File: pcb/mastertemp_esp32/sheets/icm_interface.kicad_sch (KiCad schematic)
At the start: 9 parts, among them J2 OPERATING_CONTROL_7P, K1 G5Q-1A-DC5_CANDIDATE, K2 G5Q-1A-DC5_CANDIDATE, Q1 RELAY_K1_LOW_SIDE_TBD, Q2 RELAY_K2_LOW_SIDE_TBD

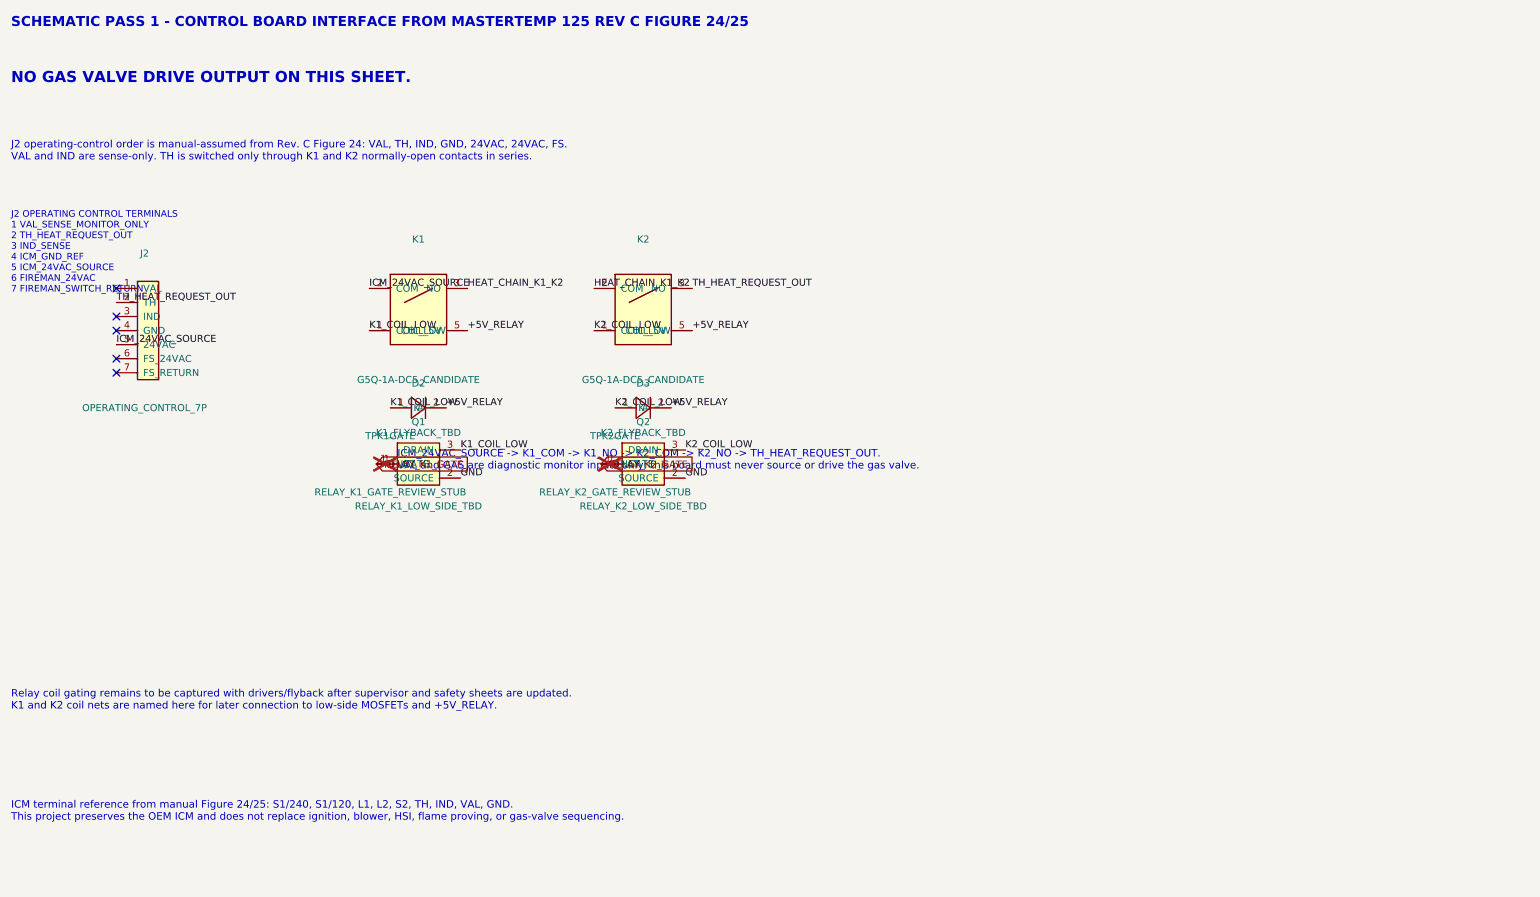
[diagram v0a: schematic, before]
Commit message: AI
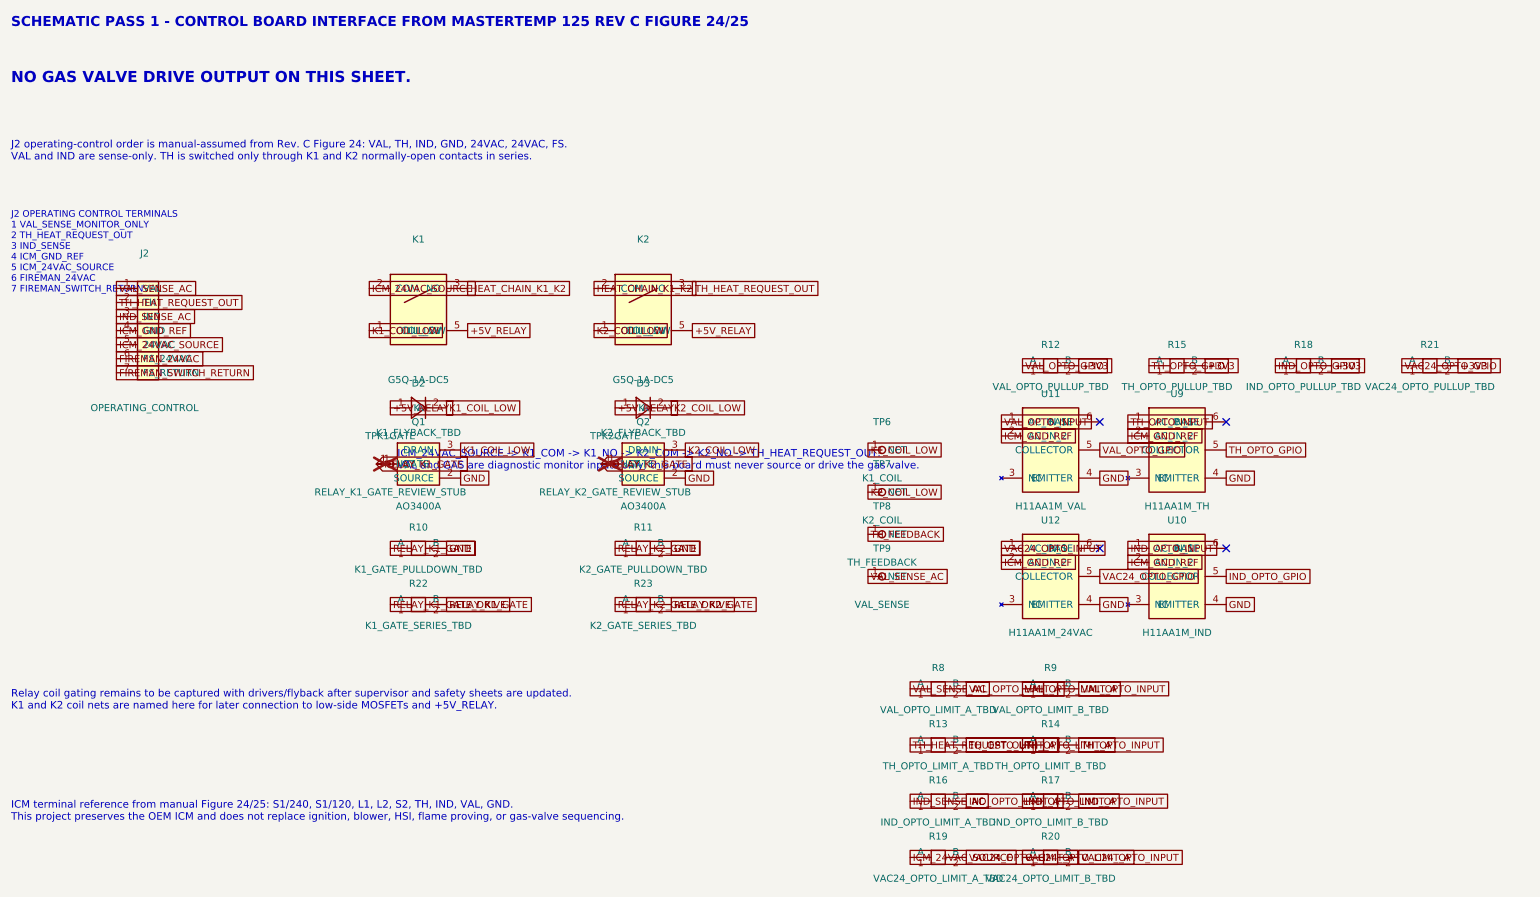
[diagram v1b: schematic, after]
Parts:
- added R10: K1_GATE_PULLDOWN_TBD, Resistor_SMD:R_0805_2012Metric, symbol mastertemp_esp32:Resistor_2pin
- added R11: K2_GATE_PULLDOWN_TBD, Resistor_SMD:R_0805_2012Metric, symbol mastertemp_esp32:Resistor_2pin
- added R12: VAL_OPTO_PULLUP_TBD, Resistor_SMD:R_0805_2012Metric, symbol mastertemp_esp32:Resistor_2pin
- added R13: TH_OPTO_LIMIT_A_TBD, Resistor_SMD:R_0805_2012Metric, symbol mastertemp_esp32:Resistor_2pin
- added R14: TH_OPTO_LIMIT_B_TBD, Resistor_SMD:R_0805_2012Metric, symbol mastertemp_esp32:Resistor_2pin
- added R15: TH_OPTO_PULLUP_TBD, Resistor_SMD:R_0805_2012Metric, symbol mastertemp_esp32:Resistor_2pin
- added R16: IND_OPTO_LIMIT_A_TBD, Resistor_SMD:R_0805_2012Metric, symbol mastertemp_esp32:Resistor_2pin
- added R17: IND_OPTO_LIMIT_B_TBD, Resistor_SMD:R_0805_2012Metric, symbol mastertemp_esp32:Resistor_2pin
- added R18: IND_OPTO_PULLUP_TBD, Resistor_SMD:R_0805_2012Metric, symbol mastertemp_esp32:Resistor_2pin
- added R19: VAC24_OPTO_LIMIT_A_TBD, Resistor_SMD:R_0805_2012Metric, symbol mastertemp_esp32:Resistor_2pin
- added R20: VAC24_OPTO_LIMIT_B_TBD, Resistor_SMD:R_0805_2012Metric, symbol mastertemp_esp32:Resistor_2pin
- added R21: VAC24_OPTO_PULLUP_TBD, Resistor_SMD:R_0805_2012Metric, symbol mastertemp_esp32:Resistor_2pin
- added R22: K1_GATE_SERIES_TBD, Resistor_SMD:R_0805_2012Metric, symbol mastertemp_esp32:Resistor_2pin
- added R23: K2_GATE_SERIES_TBD, Resistor_SMD:R_0805_2012Metric, symbol mastertemp_esp32:Resistor_2pin
- added R8: VAL_OPTO_LIMIT_A_TBD, Resistor_SMD:R_0805_2012Metric, symbol mastertemp_esp32:Resistor_2pin
- added R9: VAL_OPTO_LIMIT_B_TBD, Resistor_SMD:R_0805_2012Metric, symbol mastertemp_esp32:Resistor_2pin
- added TP6: K1_COIL, TestPoint_Pad_D2.0mm, symbol mastertemp_esp32:NetStub_1pin
- added TP7: K2_COIL, TestPoint_Pad_D2.0mm, symbol mastertemp_esp32:NetStub_1pin
- added TP8: TH_FEEDBACK, TestPoint_Pad_D2.0mm, symbol mastertemp_esp32:NetStub_1pin
- added TP9: VAL_SENSE, TestPoint_Pad_D2.0mm, symbol mastertemp_esp32:NetStub_1pin
- added U10: H11AA1M_IND, Package_DIP:DIP-6_W7.62mm, symbol mastertemp_esp32:H11AA1M
- added U11: H11AA1M_VAL, Package_DIP:DIP-6_W7.62mm, symbol mastertemp_esp32:H11AA1M
- added U12: H11AA1M_24VAC, Package_DIP:DIP-6_W7.62mm, symbol mastertemp_esp32:H11AA1M
- added U9: H11AA1M_TH, Package_DIP:DIP-6_W7.62mm, symbol mastertemp_esp32:H11AA1M
- D2, D3: footprint (none) -> Diode_SMD:D_SOD-123
- J2: value OPERATING_CONTROL_7P -> OPERATING_CONTROL; footprint Connector_Phoenix_MC_HighVoltage:PhoenixContact_MSTBA_2,5_7-G-5,08_1x07_P5.08mm_Horizontal -> Connector_Phoenix_MSTB:PhoenixContact_MSTBA_2,5_7-G-5,08_1x07_P5.08mm_Horizontal
- K1, K2: value G5Q-1A-DC5_CANDIDATE -> G5Q-1A-DC5
- Q1: value RELAY_K1_LOW_SIDE_TBD -> AO3400A
- Q2: value RELAY_K2_LOW_SIDE_TBD -> AO3400A
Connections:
- net +5V_RELAY: now also D2.1 (A), D3.1 (A); no longer D2.2 (K), D3.2 (K)
- net GND: now also R10.2 (B), R11.2 (B), U10.4 (EMITTER), U11.4 (EMITTER), U12.4 (EMITTER), U9.4 (EMITTER)
- net ICM_24VAC_SOURCE: now also R19.1 (A)
- net K1_COIL_LOW: now also D2.2 (K), TP6.1 (NET); no longer D2.1 (A)
- net K2_COIL_LOW: now also D3.2 (K), TP7.1 (NET); no longer D3.1 (A)
- net RELAY_K1_GATE: now also R10.1 (A), R22.2 (B)
- net RELAY_K2_GATE: now also R11.1 (A), R23.2 (B)
- net TH_HEAT_REQUEST_OUT: now also R13.1 (A)
- net VAL_SENSE_AC: now reaches J2.1 (VAL)
- net VAL_SENSE_AC: now also R8.1 (A), TP9.1 (NET)
- net IND_SENSE_AC: now reaches J2.3 (IND)
- net IND_SENSE_AC: now also R16.1 (A)
- net ICM_GND_REF: now reaches J2.4 (GND)
- net ICM_GND_REF: now also U10.2 (AC_IN_2), U11.2 (AC_IN_2), U12.2 (AC_IN_2), U9.2 (AC_IN_2)
- net FIREMAN_24VAC: now reaches J2.6 (FS_24VAC)
- net FIREMAN_SWITCH_RETURN: now reaches J2.7 (FS_RETURN)
- new net +3V3: R12.2 (B), R15.2 (B), R18.2 (B), R21.2 (B)
- new net IND_OPTO_GPIO: R18.1 (A), U10.5 (COLLECTOR)
- new net IND_OPTO_INPUT: R17.2 (B), U10.1 (AC_IN_1)
- new net IND_OPTO_LIMIT_A: R16.2 (B), R17.1 (A)
- new net RELAY_K1_GATE_DRIVE: R22.1 (A)
- new net RELAY_K2_GATE_DRIVE: R23.1 (A)
- new net TH_FEEDBACK: TP8.1 (NET)
- new net TH_OPTO_GPIO: R15.1 (A), U9.5 (COLLECTOR)
- new net TH_OPTO_INPUT: R14.2 (B), U9.1 (AC_IN_1)
- new net TH_OPTO_LIMIT_A: R13.2 (B), R14.1 (A)
- new net VAC24_OPTO_GPIO: R21.1 (A), U12.5 (COLLECTOR)
- new net VAC24_OPTO_INPUT: R20.2 (B), U12.1 (AC_IN_1)
- new net VAC24_OPTO_LIMIT_A: R19.2 (B), R20.1 (A)
- new net VAL_OPTO_GPIO: R12.1 (A), U11.5 (COLLECTOR)
- new net VAL_OPTO_INPUT: R9.2 (B), U11.1 (AC_IN_1)
- new net VAL_OPTO_LIMIT_A: R8.2 (B), R9.1 (A)
- no-connect marks 5 -> 4
